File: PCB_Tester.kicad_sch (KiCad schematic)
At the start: 69 parts, among them IC1 MCP4551-103E_MS, IC2 MCP4551-103E_MS, J1 Conn_01x14_Pin, J2 Conn_01x15_Pin, J3 Conn_01x04_Pin, J4 Conn_01x04_Pin, U1 ULN2003A, U2 ULN2003A

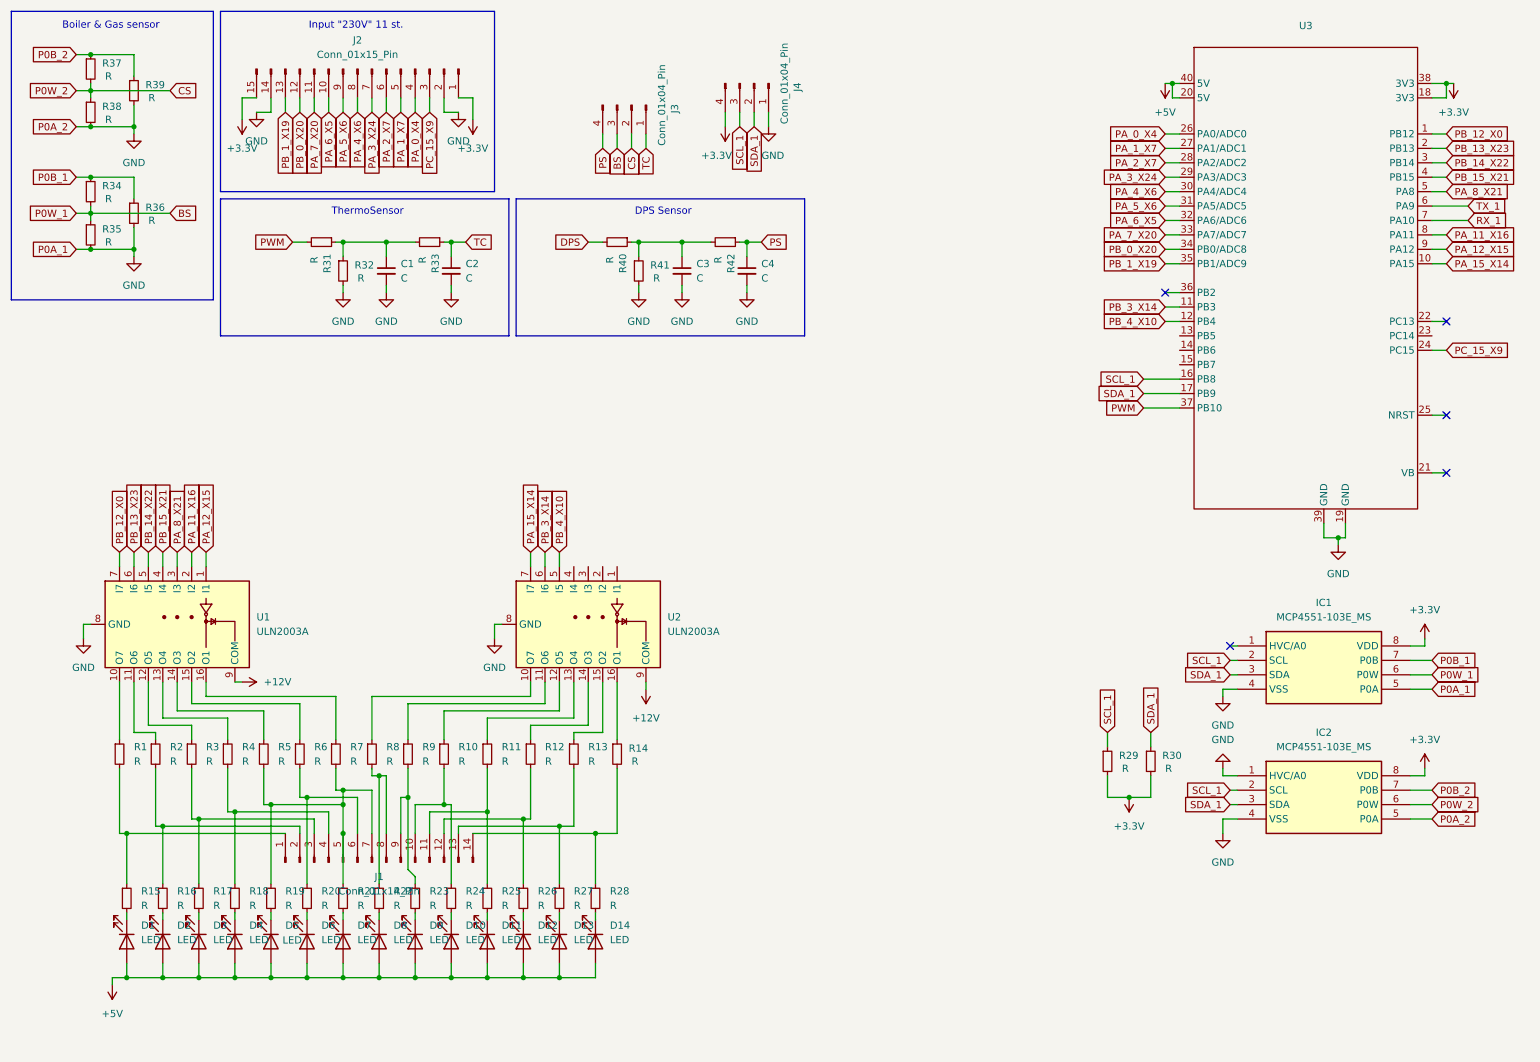
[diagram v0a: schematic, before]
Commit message: 1
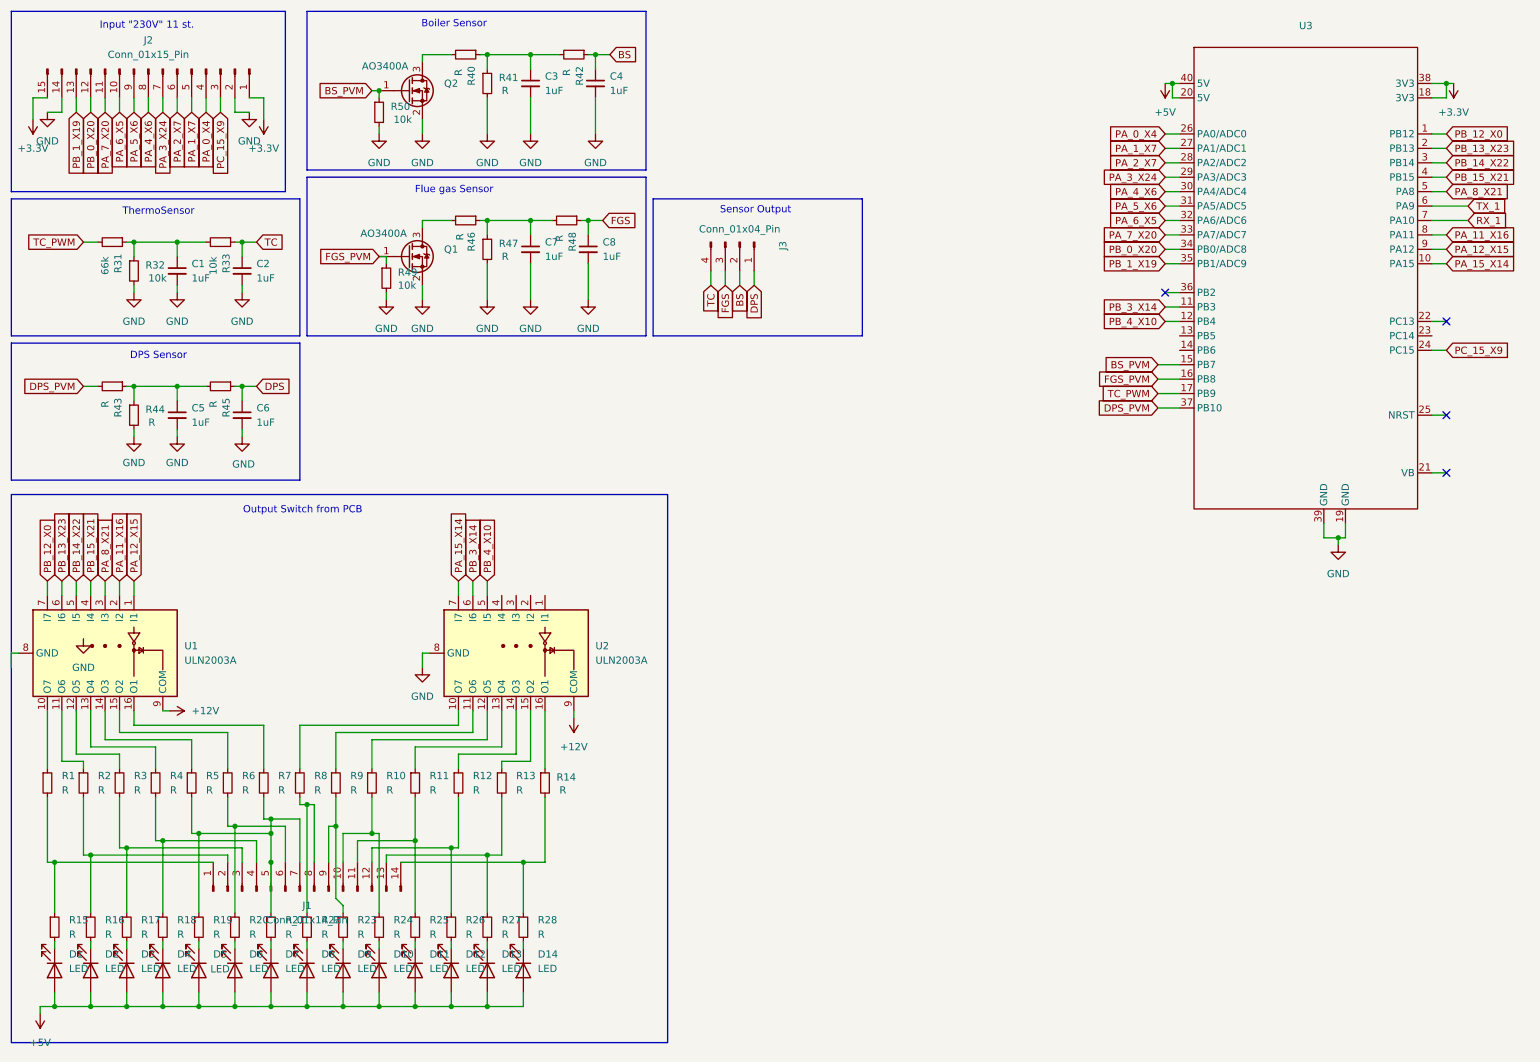
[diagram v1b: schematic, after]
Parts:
- removed IC1, IC2: MCP4551-103E_MS, Library:SOP65P490X110-8N, symbol MCP4551-103E_MS:MCP4551-103E_MS
- removed J4: Conn_01x04_Pin, Connector_PinHeader_2.54mm:PinHeader_1x04_P2.54mm_Vertical, symbol Connector:Conn_01x04_Pin
- removed R29, R30, R34, R35, R36, R37, R38, R39: R, Resistor_SMD:R_0805_2012Metric, symbol Device:R_Small
- added C5, C6, C7, C8: 1uF, Capacitor_SMD:C_0805_2012Metric, symbol Device:C_Small
- added Q1, Q2: AO3400A, Package_TO_SOT_SMD:SOT-23, symbol Transistor_FET:AO3400A
- added R43, R44, R45, R46, R47, R48: R, Resistor_SMD:R_0805_2012Metric, symbol Device:R_Small
- added R49, R50: 10k, Resistor_SMD:R_0805_2012Metric, symbol Device:R_Small
- C1, C2, C3, C4: value C -> 1uF; footprint (none) -> Capacitor_SMD:C_0805_2012Metric
- R31: value R -> 66k
- R32, R33: value R -> 10k
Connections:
- net CS is gone; now on net BS: J3.2 (Pin_2)
- net BS: now also C4.1, R42.1; no longer J3.3 (Pin_3)
- net DPS: now also J3.1 (Pin_1), C6.1, R45.1; no longer R40.2
- net GND: now also C5.2, C6.2, C7.2, C8.2, Q1.2 (S), Q2.2 (S), R44.2, R47.2, R49.2, R50.2; no longer U1.8 (GND)
- net TC: now also J3.4 (Pin_4); no longer J3.1 (Pin_1)
- net BS_PVM: now reaches U3.15 (PB7)
- net BS_PVM: now also Q2.1 (G), R50.1
- removed net PS: C4.1, J3.4 (Pin_4), R42.1
- net PWM renamed DPS_PVM
- net DPS_PVM: now also R43.2; no longer R31.2
- net SCL_1 renamed FGS_PVM
- net FGS_PVM: now also Q1.1 (G), R49.1
- net SDA_1 renamed TC_PWM
- net TC_PWM: now also R31.2
- new net: C5.1, R43.1, R44.1, R45.2
- new net: C7.1, R46.1, R47.1, R48.2
- new net: Q2.3 (D), R40.2
- new net: Q1.3 (D), R46.2
- new net FGS: C8.1, J3.3 (Pin_3), R48.1
- no-connect marks 5 -> 4
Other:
- note added: "Boiler Sensor"
- note added: "Flue gas Sensor"
- note added: "Output Switch from PCB"
- note added: "Sensor Output"
- note removed: "Boiler & Gas sensor"
- moved on the sheet: C1, C2, C3, D1, D10, D11, D12, D13, D14, D2, D3, D4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
